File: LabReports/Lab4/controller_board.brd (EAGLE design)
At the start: 185 x 33 mm, 16 parts, among them J1 JST_3PIN_GND_VDD_SIG, J2 JST_3PIN_GND_VDD_SIG, J3 JST_3PIN_GND_VDD_SIG, J4 JST_3PIN_GND_VDD_SIG, J5 GIMBAL_3PIN_MATCH_TDOCU

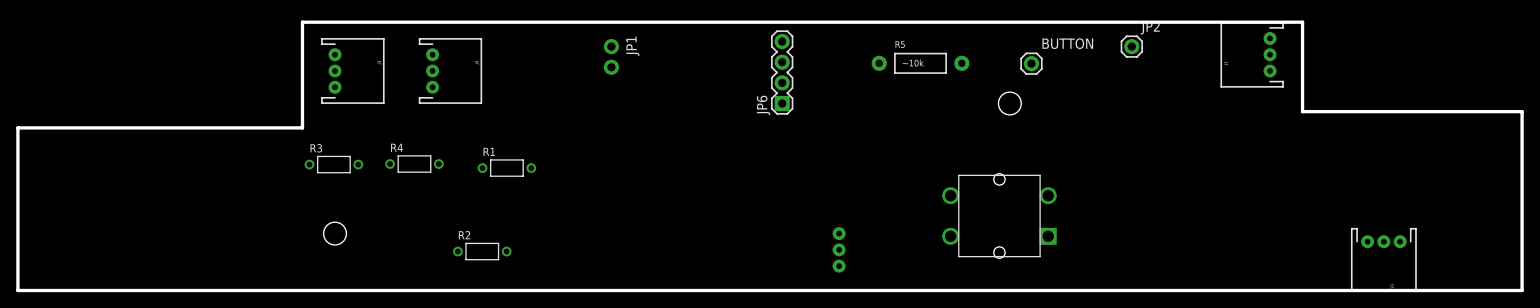
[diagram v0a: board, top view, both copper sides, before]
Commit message: Routed board and processed CAM
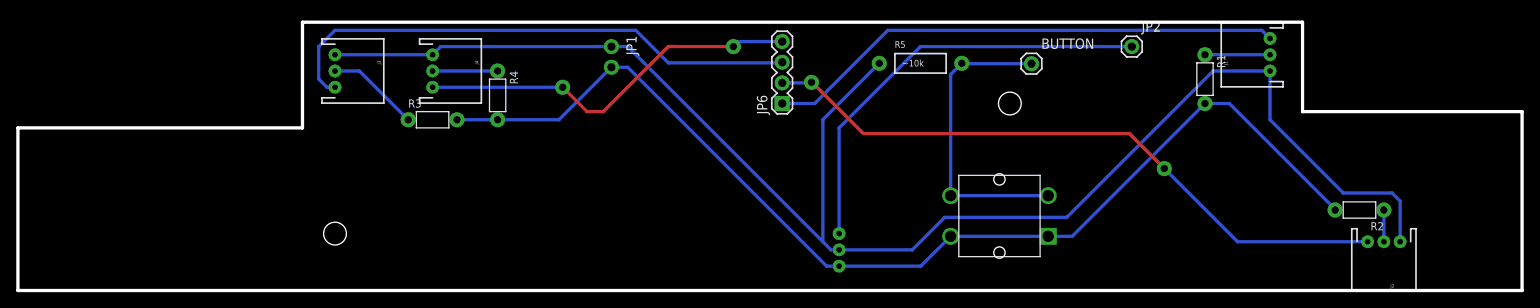
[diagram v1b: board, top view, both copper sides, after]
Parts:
- moved R2 108.0 mm to (197.0, 31.9), turned to 180 degrees
- moved R1 86.6 mm to (178.0, 48.0), turned to 270 degrees
- moved R3 13.3 mm to (83.0, 43.0)
- moved R4 13.3 mm to (91.0, 46.0), turned to 270 degrees
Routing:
- net GND: track 0.00 -> 190.8 mm
- net 3.3V: track 0.00 -> 134.5 mm
- net ROLL: track 0.00 -> 80.1 mm, vias 0 -> 2
- net THROTTLE: track 0.00 -> 66.0 mm
- net PITCH: track 0.00 -> 64.1 mm
- net N$9: track 0.00 -> 53.1 mm
- net YAW: track 0.00 -> 47.8 mm, vias 0 -> 2
- net N$6: track 0.00 -> 37.4 mm
- net N$3: track 0.00 -> 11.5 mm
- net N$4: track 0.00 -> 8.00 mm
- net N$1: track 0.00 -> 8.00 mm
- net N$2: track 0.00 -> 3.90 mm
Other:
- board text added: "CSE 190 Spring 2015"
- board text added: "Controller Board r1"
- board text added: "Trevor Smith"
